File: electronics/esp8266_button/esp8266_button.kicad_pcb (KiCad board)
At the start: 2 copper layers, 34.3 x 50.8 mm, 30 parts, among them J1 CONN_01X03, J2 CONN_01X08, J3 CONN_01X08, M1 BMP180_Breakout, P1 SYMBOL, Q1 Q_NMOS_GSD, Q2 Q_PMOS_GSD, SW1 SW_Push, SW2 SW_Push, SW3 SW_Push, U1 MCP1703A-3302/MB, U2 ESP-12

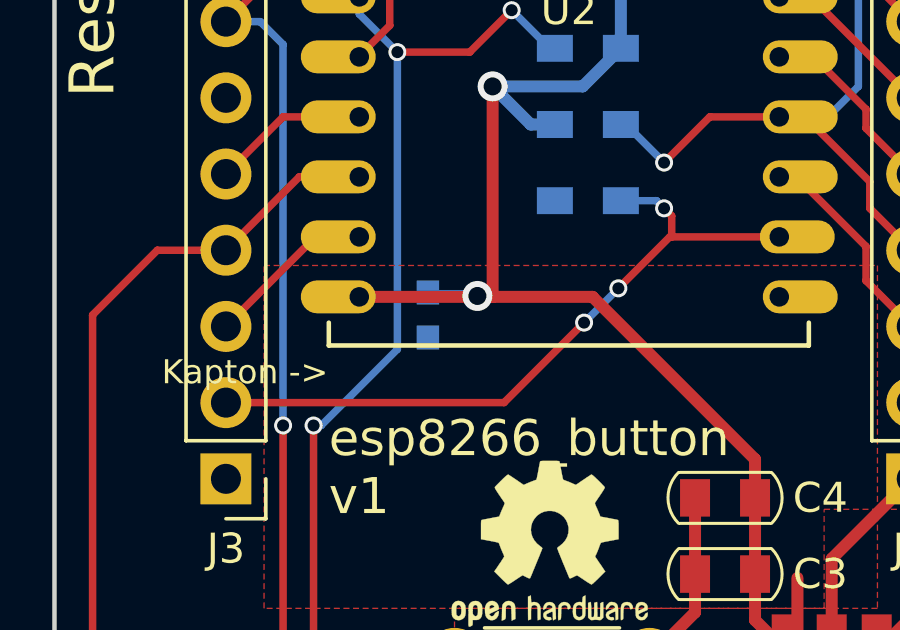
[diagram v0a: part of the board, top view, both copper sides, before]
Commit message: sync
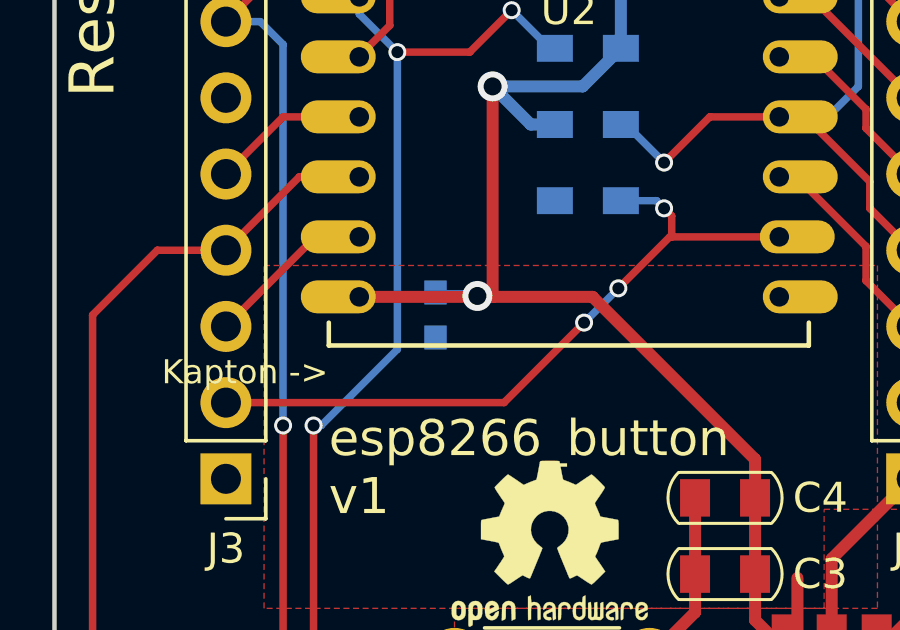
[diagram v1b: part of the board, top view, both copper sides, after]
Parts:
- moved C5 0.25 mm to (149.9, 101.6)
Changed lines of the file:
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@@
     (pad_to_mask_clearance 0.2)
     (aux_axis_origin 0 0)
-    (visible_elements FFFFFF1F)
+    (visible_elements FFFFFF5F)
     (pcbplotparams
       (layerselection 0x00030_80000001)
@@
   )
   (module Capacitors_SMD_Round:C_0603 (layer B.Cu)
-    (at 149.606 101.6 270)
+    (at 149.86 101.6 270)
     (descr "Capacitor SMD 0603, reflow soldering, AVX (see smccp.pdf)")
     (tags "capacitor 0603")
@@
   (segment (start 161.568 112.828) (end 160.512 111.772) (width 0.4) (layer F.Cu) (net 3))
   (segment (start 160.512 111.772) (end 160.512 110.236) (width 0.4) (layer F.Cu) (net 3))
-  (segment (start 149.606 100.85) (end 149.721 100.965) (width 0.4) (layer B.Cu) (net 3) (status 30))
-  (segment (start 149.721 100.965) (end 151.257 100.965) (width 0.4) (layer B.Cu) (net 3) (status 10))
+  (segment (start 149.86 100.85) (end 149.975 100.965) (width 0.4) (layer B.Cu) (net 3) (status 30))
+  (segment (start 149.975 100.965) (end 151.257 100.965) (width 0.4) (layer B.Cu) (net 3) (status 10))
   (via (at 151.257 100.965) (size 1) (drill 0.6) (layers F.Cu B.Cu) (net 3))
   (segment (start 151.257 100.965) (end 151.257 100.995) (width 0.4) (layer F.Cu) (net 3))
@@
   (segment (start 151.765 93.98) (end 153.035 95.25) (width 0.4) (layer B.Cu) (net 3))
   (via (at 151.765 93.98) (size 1) (drill 0.6) (layers F.Cu B.Cu) (net 3))
-  (segment (start 149.461 100.995) (end 149.606 100.85) (width 0.4) (layer B.Cu) (net 3) (status 30))
+  (segment (start 149.715 100.995) (end 149.86 100.85) (width 0.4) (layer B.Cu) (net 3) (status 30))
   (segment (start 160.512 107.696) (end 160.512 106.41) (width 0.4) (layer F.Cu) (net 3))
   (segment (start 155.097 100.995) (end 151.765 100.995) (width 0.4) (layer F.Cu) (net 3))
@@
   (segment (start 145.861 98.995) (end 142.875 101.981) (width 0.25) (layer F.Cu) (net 17))
   (segment (start 138.43 115.74) (end 138.43 101.6) (width 0.25) (layer F.Cu) (net 18))
+  (segment (start 138.43 101.6) (end 140.589 99.441) (width 0.25) (layer F.Cu) (net 18))
   (segment (start 140.589 99.441) (end 142.875 99.441) (width 0.25) (layer F.Cu) (net 18))
-  (segment (start 138.43 101.6) (end 140.589 99.441) (width 0.25) (layer F.Cu) (net 18))
   (segment (start 147.32 96.995) (end 145.321 96.995) (width 0.25) (layer F.Cu) (net 18))
   (segment (start 145.321 96.995) (end 142.875 99.441) (width 0.25) (layer F.Cu) (net 18))
